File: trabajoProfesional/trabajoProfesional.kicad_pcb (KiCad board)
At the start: 2 copper layers, 47 parts, among them T1 MPMOS, U1 1501

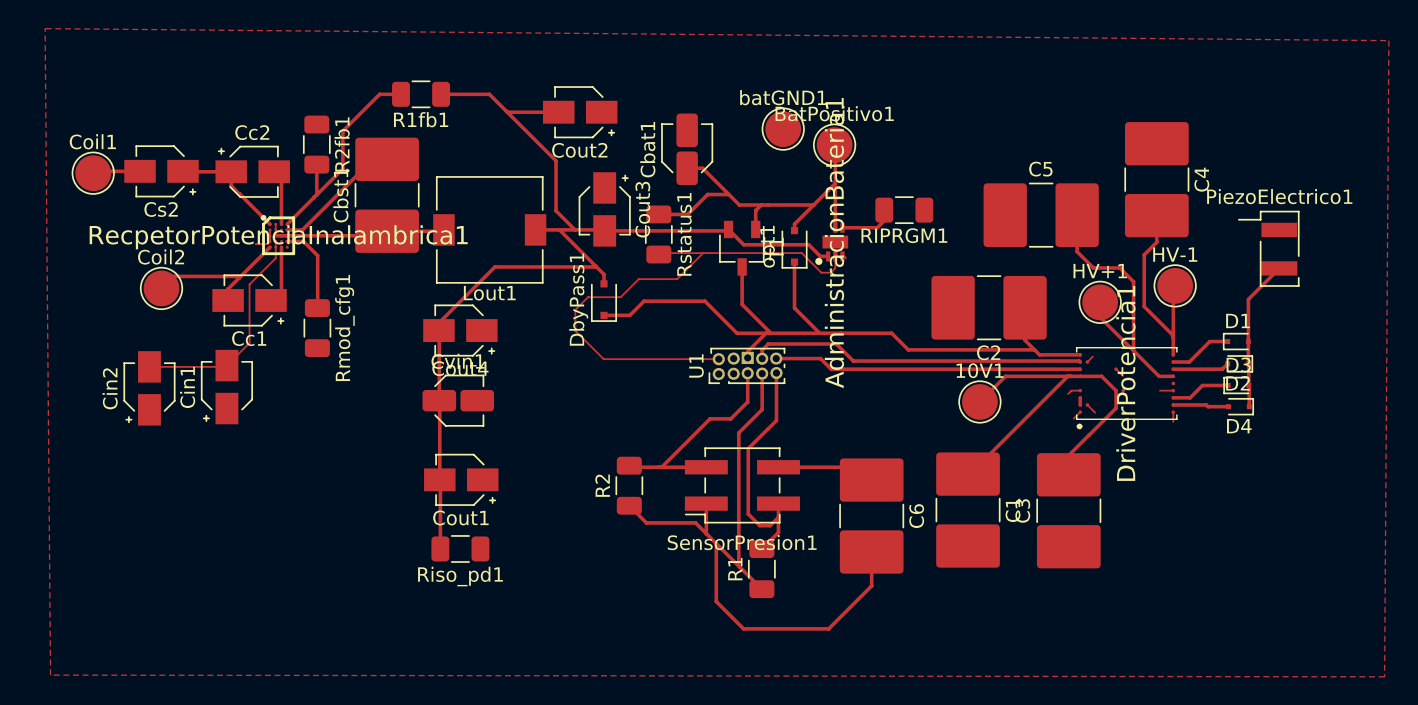
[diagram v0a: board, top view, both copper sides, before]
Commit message: va el circuito
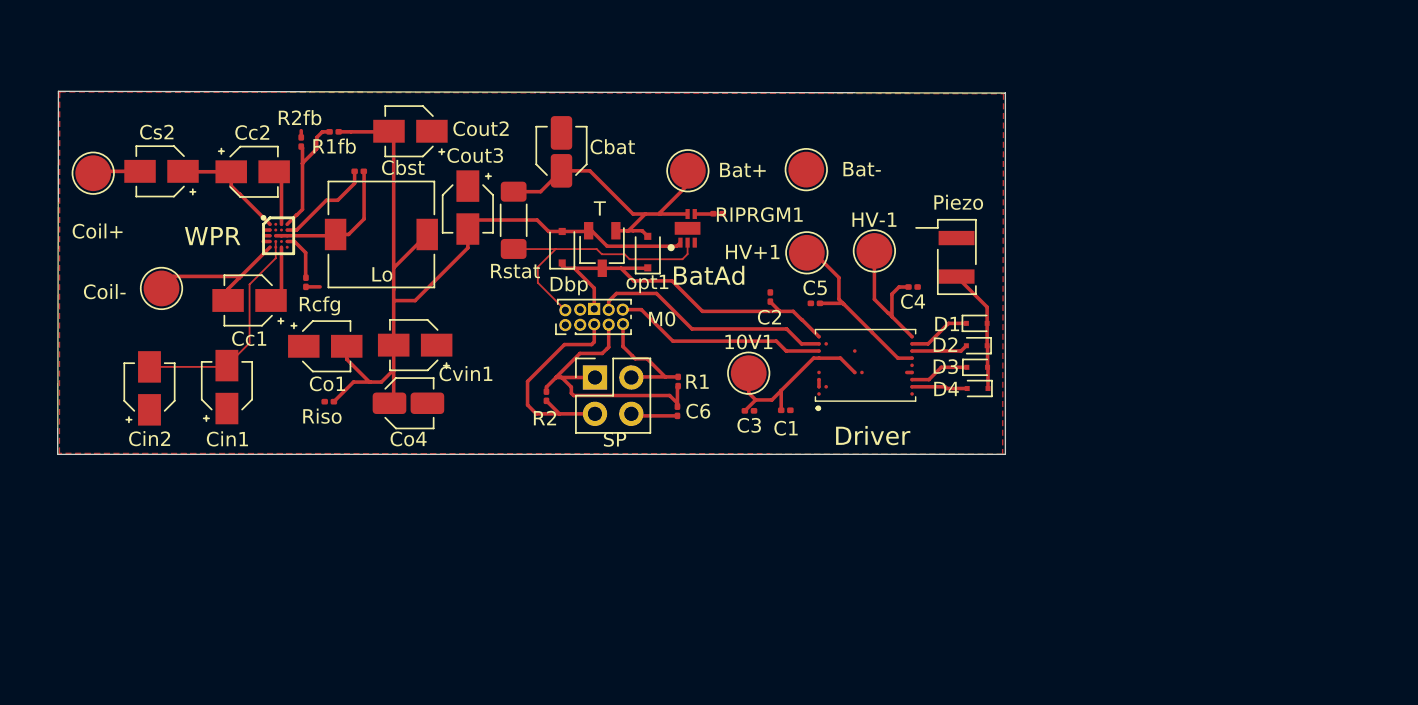
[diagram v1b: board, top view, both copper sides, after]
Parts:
- removed AdministracionBateria1: SC810ULTRT, SC810:SON50P200X200X60-7N-D
- removed Coil1: Conn_01x01_Male, TestPoint:TestPoint_Pad_D2.5mm
- removed Rstatus1: R, Resistor_SMD:R_1206_3216Metric
- added BatAd: SC810ULTRT, SC810:SON50P200X200X60-7N-D, F.Cu at (102.3, 68.7)
- added Coil+: Conn_01x01_Male, TestPoint:TestPoint_Pad_D2.5mm, F.Cu at (60.8, 64.8)
- added Rstat: R, Resistor_SMD:R_1806_4516Metric, F.Cu at (90.2, 68.1)
- C1, C2, C3, C4, C5, C6: footprint Capacitor_SMD:C_2816_7142Metric -> Capacitor_SMD:C_0201_0603Metric
- Cbst: renamed from Cbst1; footprint Capacitor_SMD:C_2816_7142Metric -> Capacitor_SMD:C_0201_0603Metric
- R1, R2, RIPRGM1: footprint Resistor_SMD:R_1206_3216Metric -> Resistor_SMD:R_0201_0603Metric
- R1fb: renamed from R1fb1; footprint Resistor_SMD:R_1206_3216Metric -> Resistor_SMD:R_0201_0603Metric
- R2fb: renamed from R2fb1; footprint Resistor_SMD:R_1206_3216Metric -> Resistor_SMD:R_0201_0603Metric
- Rcfg: renamed from Rmod_cfg1; footprint Resistor_SMD:R_1206_3216Metric -> Resistor_SMD:R_0201_0603Metric
- Riso: renamed from Riso_pd1; footprint Resistor_SMD:R_1206_3216Metric -> Resistor_SMD:R_0201_0603Metric
- SP: renamed from SensorPresion1; footprint Connector_PinSocket_2.54mm:PinSocket_2x02_P2.54mm_Vertical_SMD -> Connector_PinHeader_2.54mm:PinHeader_2x02_P2.54mm_Vertical
- moved C3 23.4 mm to (106.7, 81.4), turned to 180 degrees
- moved Piezo 22.6 mm to (121.2, 70.7)
- moved HV-1 21.2 mm to (115.4, 70.2)
- moved HV+1 20.8 mm to (110.7, 70.4)
- moved C4 18.6 mm to (118.1, 72.8), turned to 180 degrees
- moved D4 18.3 mm to (122.6, 79.8)
- moved D1 18.3 mm to (122.5, 75.3)
- moved D2 18.3 mm to (122.5, 76.9)
- moved D3 18.3 mm to (122.6, 78.4)
- moved Driver 18.3 mm to (114.8, 78.2)
- moved C5 16.9 mm to (111.3, 73.9)
- moved 10V1 16.3 mm to (106.6, 78.8)
- moved C6 15.4 mm to (101.6, 81.4), turned to 90 degrees
- moved C2 15.3 mm to (108.1, 73.5), turned to 90 degrees
- moved C1 14.5 mm to (109.2, 81.4), turned to 0 degrees
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- renumbered BatPositivo1 to Bat+, batGND1 to Bat-, Cbat1 to Cbat, Cout1 to Co1, Cout4 to Co4, Coil2 to Coil-, DbyPass1 to Dbp, DriverPotencia1 to Driver, Lout1 to Lo, U1 to M0, PiezoElectrico1 to Piezo, T1 to T, RecpetorPotenciaInalambrica1 to WPR
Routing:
- net Net-(C6-Pad2): track 47.3 -> 20.9 mm
- net /Salida/Alimentacion: track 51.9 -> 26.4 mm
- net /Bateria/Cargando: track 36.8 -> 19.0 mm
- net Net-(AdministracionBateria1-Pad1): track 73.8 -> 58.4 mm
- net 10V: track 27.9 -> 13.1 mm
- net SDAPresion: track 17.0 -> 8.70 mm
- net +HV: track 20.1 -> 13.0 mm
- net /Salida/SN1ONOFF: track 21.5 -> 14.9 mm
- net /Salida/SP1ONOFF: track 23.5 -> 17.0 mm
- net Net-(R1fb1-Pad2): track 15.3 -> 9.23 mm
- net +Bat: track 27.5 -> 22.0 mm
- net -HV: track 14.6 -> 10.0 mm
- net GND: track 7.33 -> 3.13 mm
- net Net-(C6-Pad1): track 6.88 -> 3.28 mm
- net Net-(RecpetorPotenciaInalambrica1-PadD4): track 6.21 -> 3.37 mm
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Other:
- board outline added: 66.2 x 25.4 mm
